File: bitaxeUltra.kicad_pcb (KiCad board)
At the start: 4 copper layers, 56.5 x 99.8 mm, 137 parts, among them J1 54-00164, J2 Conn_01x02, J3 Conn_01x05, J4 Conn_01x04, J5 TC2030-IDC, J7 Conn_01x02, J8 USB_C_Receptacle_USB2.0, J9 Conn_01x04, Q1 CSD17311Q5, Q2 CSD17311Q5, Q4 2N7002K, SW1 GT-TC029B-H025-L1N, SW2 GT-TC029B-H025-L1N, U1 25MHz, U10 DS4432U+, U11 RT9080-33GJ5, U12 ESP32-S3-WROOM-1, U14 BM1366_mode1, U2 TXB0104RGYR, U5 MCP1824T-1802E, U6 MCP1824T-0802E, U7 EMC2101, U8 INA260, U9 TPS40305, Y1 32.768kHz

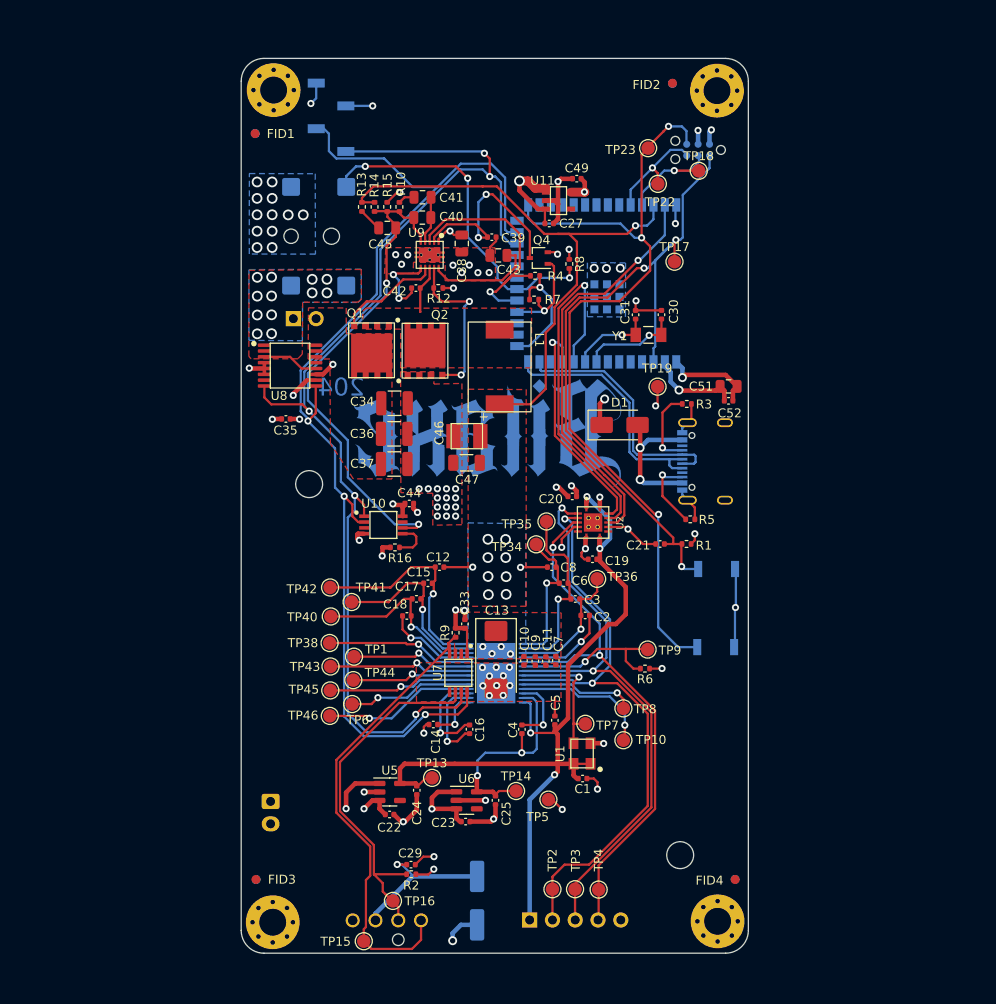
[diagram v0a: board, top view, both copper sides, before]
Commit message: Add files via upload
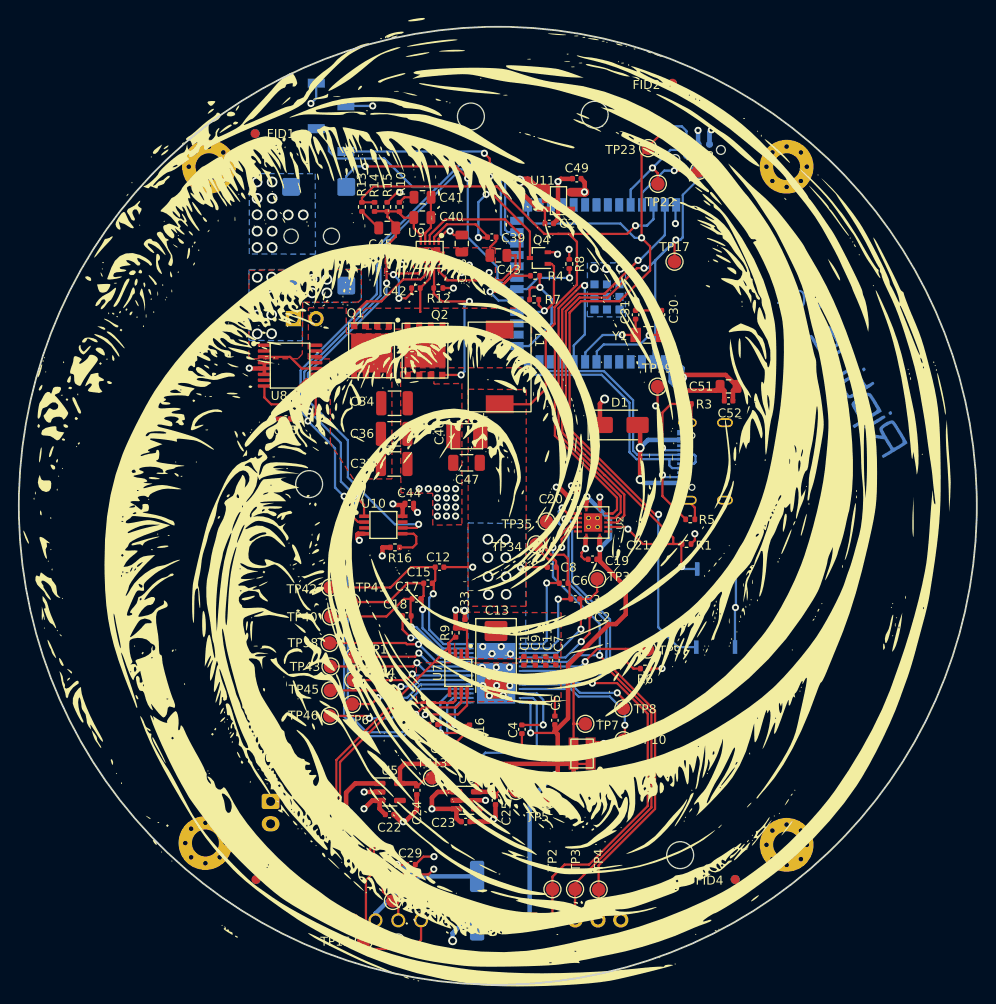
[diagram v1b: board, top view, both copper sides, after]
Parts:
- removed the G*** at (105.1, 89.7) (x2)
- added ?: , , F.Cu at (102.8, 54.0)
- added ?: , , F.Cu at (116.6, 53.8)
- added G***: LOGO, bitaxe:silk, F.Cu at (103.8, 96.3)
- added G***: LOGO, bitaxe:silk, B.Cu at (106.4, 96.2)
- added G*** (x2): LOGO, bitaxe:words, B.Cu at (146.0, 84.6)
- moved H10 11.6 mm to (73.2, 135.0)
- moved H7 11.5 mm to (138.0, 59.6)
- moved H9 11.5 mm to (138.0, 135.2)
- moved H8 11.2 mm to (73.6, 59.6)
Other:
- board size 56.5 x 99.8 mm -> 106.8 x 106.8 mm
